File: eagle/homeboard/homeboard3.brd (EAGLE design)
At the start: 100 x 80 mm, 81 parts, among them IC1 XCF02S, IC2 25LC080SN, Q5 BC848SMD, Q6 BC848SMD, Q7 BC848SMD, Q8 BC848SMD, T1 BSS138, T2 BC848, T3 BSS138, U1 XC3S400TQ144, X1 1503_04, X2 SCART-F

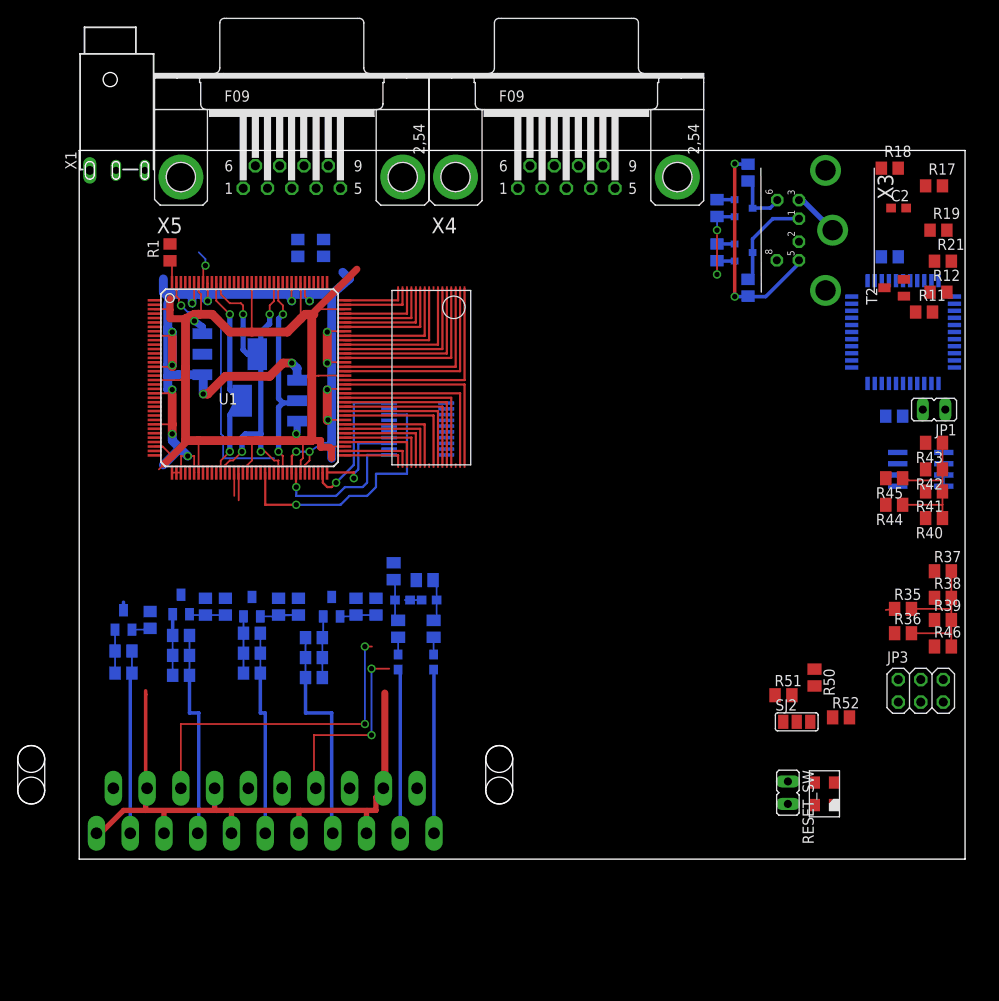
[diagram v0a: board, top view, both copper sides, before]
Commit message: rough positioning
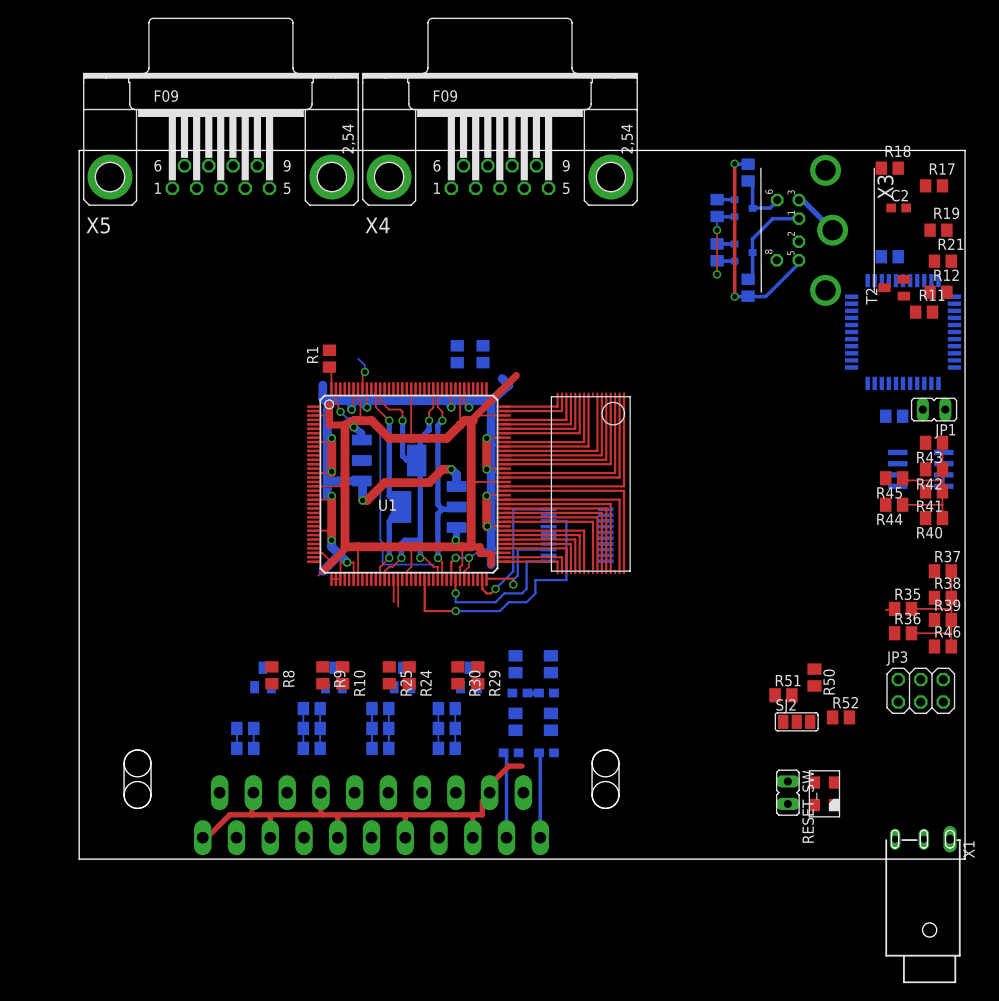
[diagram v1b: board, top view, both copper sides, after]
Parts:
- moved X1 133.3 mm to (96.0, -8.00), turned to 180 degrees
- moved IC1 21.6 mm to (59.1, 39.5)
- moved R1 21.6 mm to (28.2, 56.5)
- moved R2 21.6 mm to (45.6, 57.0)
- moved R3 21.6 mm to (42.7, 57.0)
- moved REG1.2 21.6 mm to (35.0, 45.0)
- moved REG2.5 21.6 mm to (39.5, 39.8)
- moved U$1 21.6 mm to (57.8, 42.7)
- moved U1 21.6 mm to (37.2, 42.3)
- moved Q6 19.1 mm to (28.8, 20.5)
- moved Q8 18.8 mm to (36.5, 20.5)
- moved Q7 17.4 mm to (44.0, 20.5)
- moved R10 17.3 mm to (29.8, 20.8), flipped to the top
- moved R23 17.3 mm to (49.2, 22.0)
- moved R34 17.1 mm to (53.2, 22.0), turned to 270 degrees
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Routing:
- net SCART_BLANKING: track 37.6 -> 0.00 mm, vias 2 -> 0
- net SCART_MODE: track 22.5 -> 0.00 mm, vias 2 -> 0
- net SCART_BLUE: track 25.1 -> 4.67 mm
- net SCART_RED: track 23.4 -> 4.50 mm
- net SCART_GREEN: track 23.1 -> 4.50 mm
- net SCART_COMP: track 20.7 -> 2.25 mm
- net GND: track 234.3 -> 217.0 mm
- net SCART_LEFT: track 18.6 -> 9.72 mm
- net SCART_RIGHT: track 18.5 -> 9.64 mm
- net N$55: track 6.59 -> 0.00 mm
- net N$51: track 4.78 -> 0.00 mm
- net N$65: track 4.89 -> 0.49 mm
- net N$57: track 4.20 -> 0.00 mm
- net N$53: track 4.15 -> 0.00 mm
- net N$59: track 4.90 -> 2.25 mm
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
